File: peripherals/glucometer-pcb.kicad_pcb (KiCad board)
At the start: 2 copper layers, 46.1 x 72.7 mm, 10 parts, among them U1 ESP32_DevKit_V1_DOIT

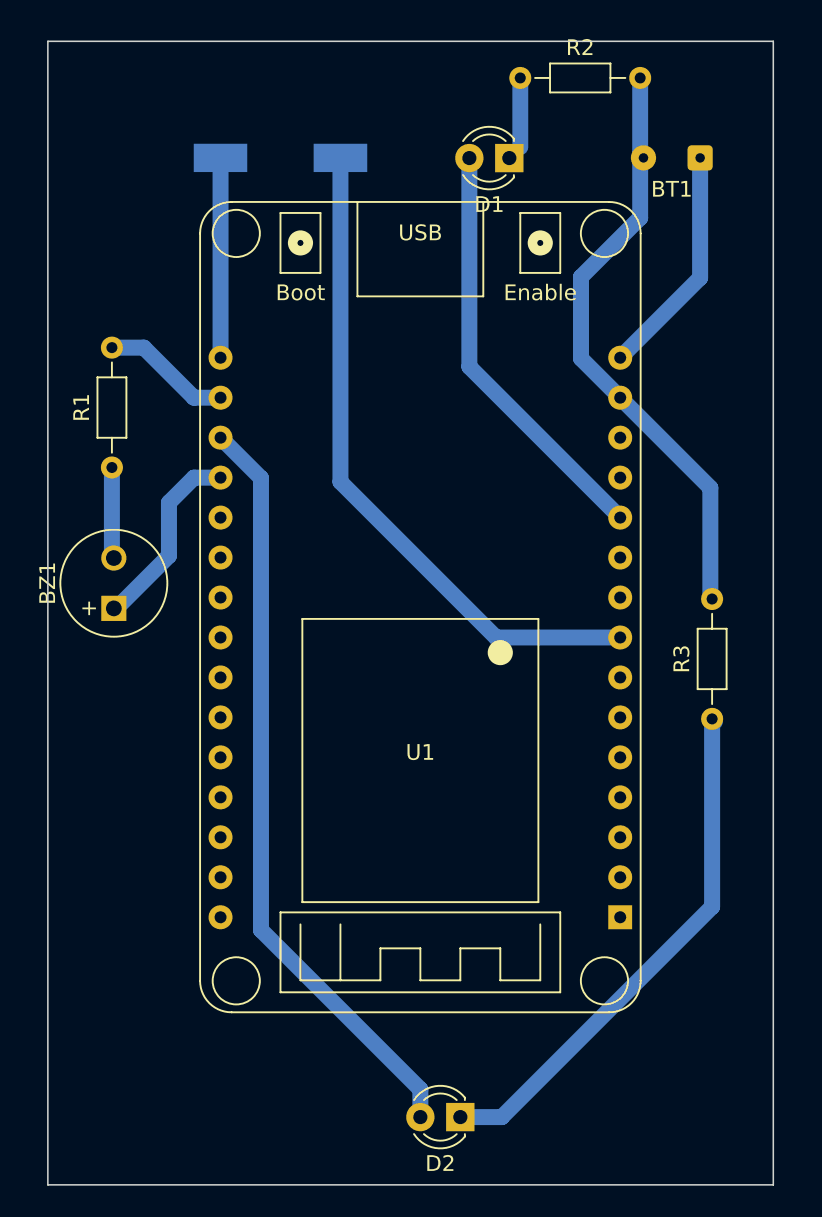
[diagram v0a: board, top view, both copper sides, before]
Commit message: fixed PCB
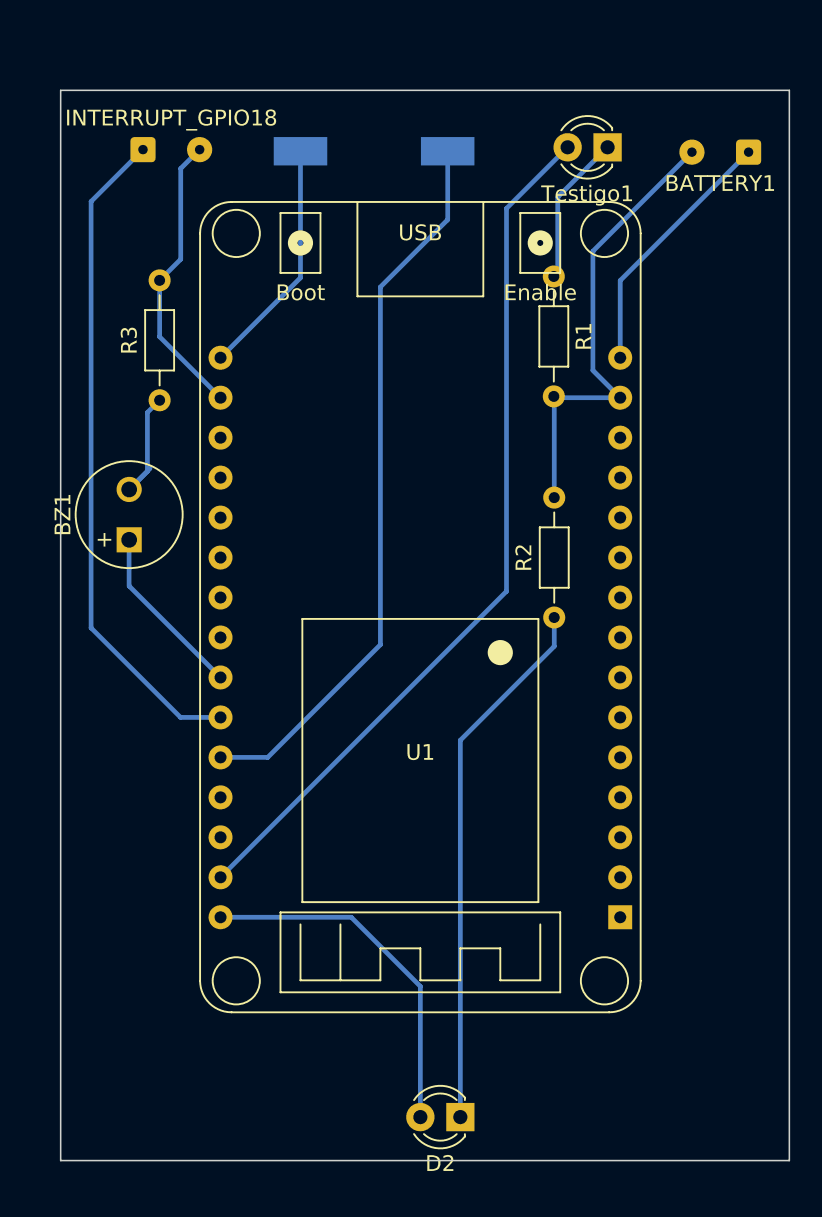
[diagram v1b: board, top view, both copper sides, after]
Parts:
- added INTERRUPT_GPIO18: SW_Push, Connector_Wire:SolderWire-0.1sqmm_1x02_P3.6mm_D0.4mm_OD1mm, F.Cu at (190.7, 70.6)
- moved R1 12.8 mm to (216.8, 78.7), turned to -90 degrees
- moved R2 11.9 mm to (216.8, 100.3)
- moved SIGNAL_IN1 6.83 mm to (210.0, 70.7)
- moved Testigo1 6.28 mm to (220.2, 70.4)
- moved R3 5.24 mm to (191.7, 86.5)
- moved 3V3_OUT1 5.10 mm to (200.7, 70.7)
- moved BZ1 4.47 mm to (189.8, 95.4)
- moved BATTERY1 3.10 mm to (229.1, 70.8)
- renumbered BT1 to BATTERY1, R2 to R1, R3 to R2, R1 to R3, TP1 to SIGNAL_IN1, D1 to Testigo1
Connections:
- BZ1 pad 1: Net-(BZ1-Pad1) -> Net-(U1-Pad24)
- D2 pad 2: Net-(D2-Pad2) -> Net-(U1-Pad30)
- SIGNAL_IN1 pad 1: SIGNAL_OUT -> Net-(SIGNAL_IN1-Pad1)
- Testigo1 pad 2: Net-(D1-Pad2) -> Net-(U1-Pad29)
- U1 pad 11: Net-(D1-Pad2) -> unconnected-(U1-Pad11)
- U1 pad 18: Net-(D2-Pad2) -> unconnected-(U1-Pad18)
- U1 pad 19: Net-(BZ1-Pad1) -> unconnected-(U1-Pad19)
- U1 pad 24: unconnected-(U1-Pad24) -> Net-(U1-Pad24)
- U1 pad 25: unconnected-(U1-Pad25) -> Net-(U1-Pad25)
- U1 pad 26: unconnected-(U1-Pad26) -> Net-(SIGNAL_IN1-Pad1)
- U1 pad 29: unconnected-(U1-Pad29) -> Net-(U1-Pad29)
- U1 pad 30: unconnected-(U1-Pad30) -> Net-(U1-Pad30)
- U1 pad 8: SIGNAL_OUT -> unconnected-(U1-Pad8)
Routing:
- net Net-(U1-Pad29): track 0.00 -> 56.5 mm
- net Net-(D2-Pad2): track 48.4 -> 0.00 mm
- net Net-(SIGNAL_IN1-Pad1): track 0.00 -> 46.3 mm
- net SIGNAL_OUT: track 42.5 -> 0.00 mm
- net Net-(U1-Pad25): track 0.00 -> 42.3 mm
- net Net-(D1-Pad2): track 26.8 -> 0.00 mm
- net Net-(U1-Pad30): track 0.00 -> 22.8 mm
- net Net-(BZ1-Pad1): track 12.2 -> 0.00 mm
- net Net-(U1-Pad24): track 0.00 -> 11.2 mm
- net Net-(Testigo1-Pad1): track 5.38 -> 9.27 mm
- net Net-(BZ1-Pad2): track 5.80 -> 8.35 mm
- net VCC: track 12.7 -> 15.2 mm
- net GND: track 46.6 -> 48.4 mm
- net Net-(BATTERY1-Pad1): track 14.8 -> 16.4 mm
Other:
- board size 46.1 x 72.7 mm -> 46.3 x 68 mm
